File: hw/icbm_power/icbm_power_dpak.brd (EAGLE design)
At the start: 21.6 x 68.6 mm, 26 parts

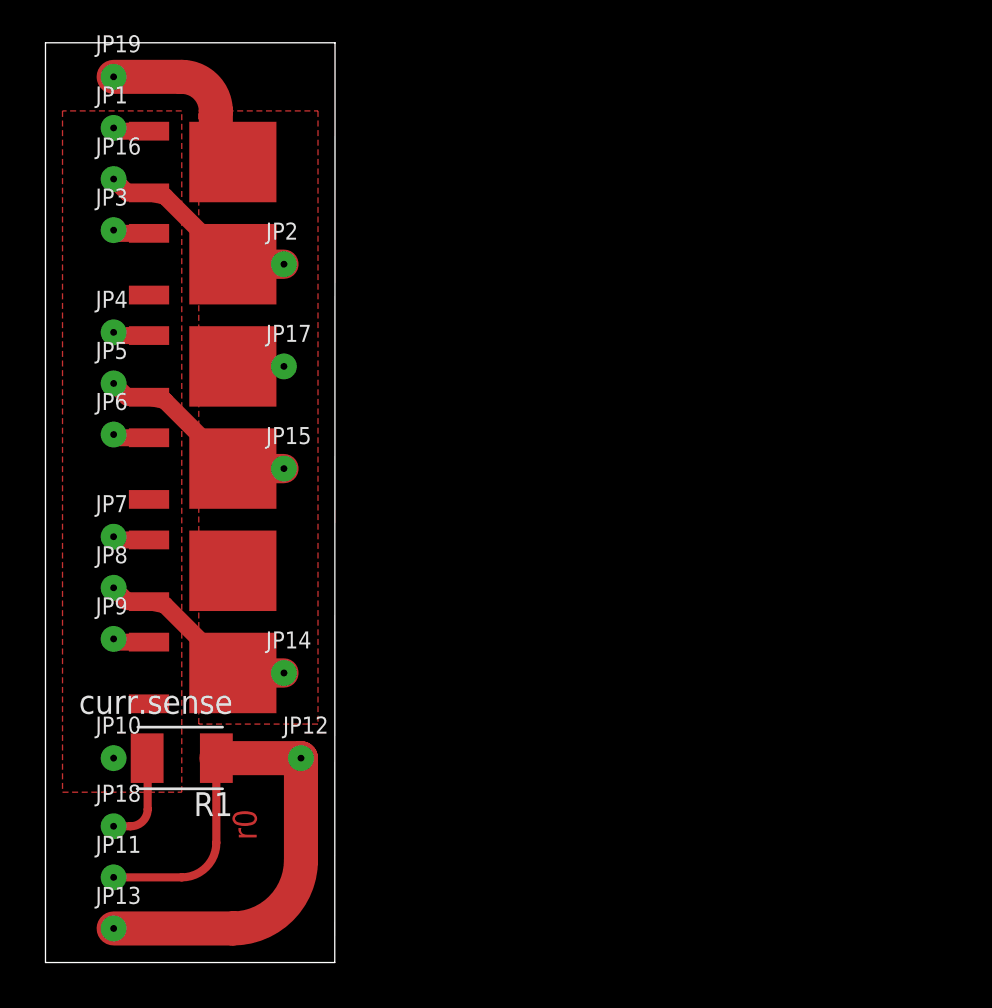
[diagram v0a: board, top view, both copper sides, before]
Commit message: oldie sync
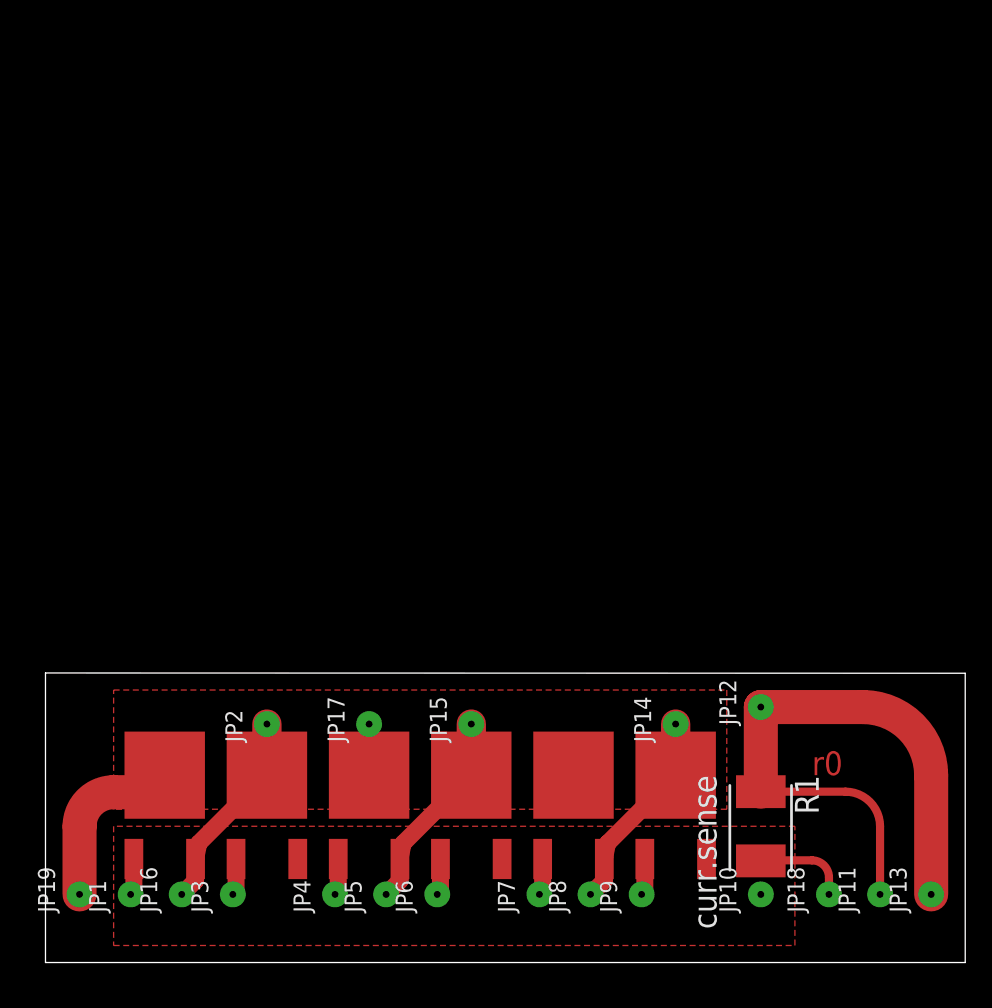
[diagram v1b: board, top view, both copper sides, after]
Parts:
- moved JP13 61.0 mm to (66.0, 5.08), turned to 90 degrees
- moved JP19 61.0 mm to (2.54, 5.08), turned to 90 degrees
- moved JP1 57.2 mm to (6.35, 5.08), turned to 90 degrees
- moved JP11 57.2 mm to (62.2, 5.08), turned to 90 degrees
- moved JP16 53.6 mm to (10.2, 5.08), turned to 90 degrees
- moved JP18 53.6 mm to (58.4, 5.08), turned to 90 degrees
- moved JP3 50.3 mm to (14.0, 5.08), turned to 90 degrees
- moved JP10 49.3 mm to (53.3, 5.08), turned to 90 degrees
- moved Q1 46.0 mm to (8.89, 14.0), turned to 0 degrees
- moved JP4 45.0 mm to (21.6, 5.08), turned to 90 degrees
- moved JP9 43.7 mm to (44.5, 5.08), turned to 90 degrees
- moved R1 43.5 mm to (53.3, 10.2), turned to 270 degrees
- moved JP5 43.2 mm to (25.4, 5.08), turned to 90 degrees
- moved JP8 42.3 mm to (40.6, 5.08), turned to 90 degrees
- moved JP6 41.9 mm to (29.2, 5.08), turned to 90 degrees
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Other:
- board size 21.6 x 68.6 mm -> 68.6 x 21.6 mm
